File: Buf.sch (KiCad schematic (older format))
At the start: 24 parts, among them U13 74AHCT573, U15 74AHCT573, U16 74AHCT573, U17 74AHCT573, U18 74AHCT573, U19 74AHCT573, U2 74AHCT573, U20 74AHCT573, U21 74AHCT573, U22 74AHCT573, U23 74AHCT573, U24 74AHCT573

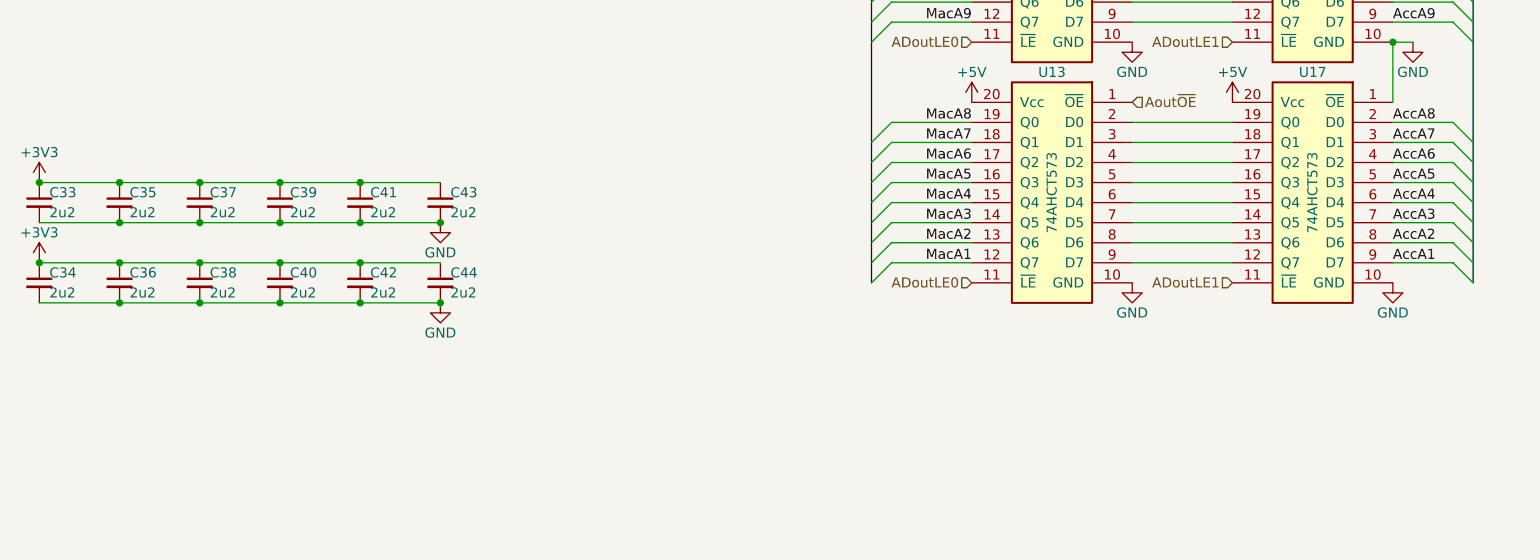
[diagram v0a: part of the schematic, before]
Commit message: Add LC... sloppy
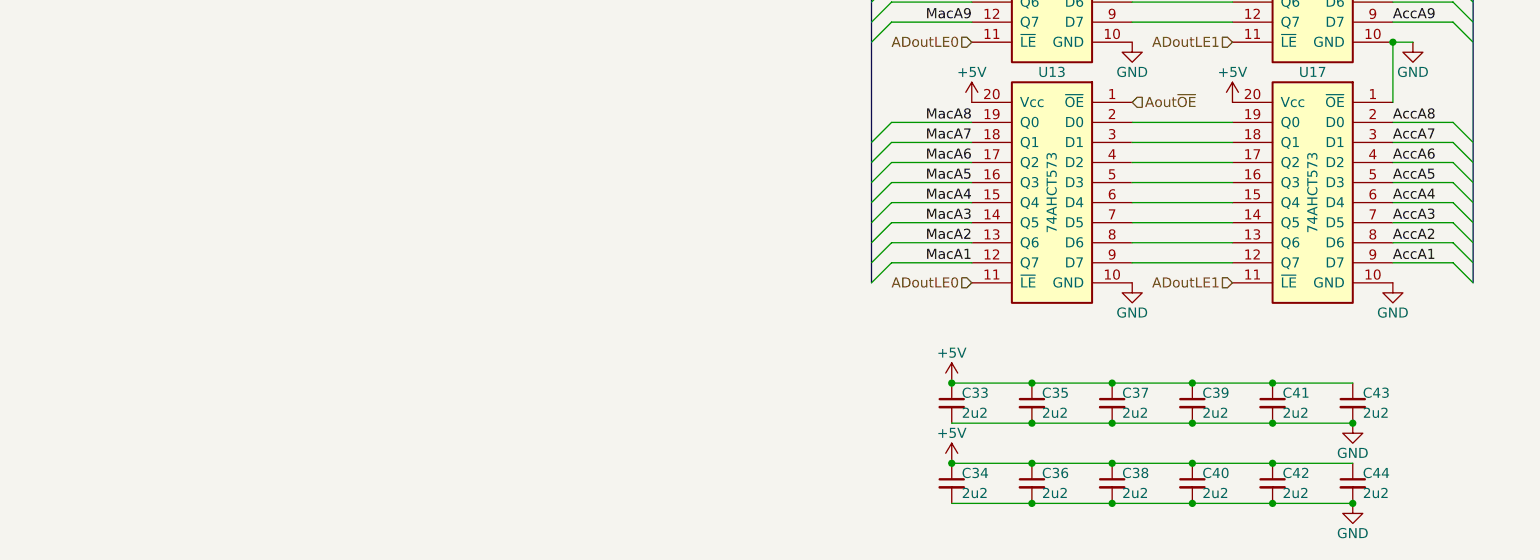
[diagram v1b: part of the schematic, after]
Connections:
- net +3V3 is gone; now on net +5V: C33.1, C34.1, C35.1, C36.1, C37.1, C38.1, C39.1, C40.1, C41.1, C42.1, C43.1, C44.1
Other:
- moved on the sheet: C33, C34, C35, C36, C37, C38, C39, C40, C41, C42, C43, C44
